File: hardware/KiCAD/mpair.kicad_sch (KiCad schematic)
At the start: 26 parts, among them J3 DX07S016JA1R1500, J4 ARJP11A-MASA-B-A-EMU2, U1 USBLC6-2SC6

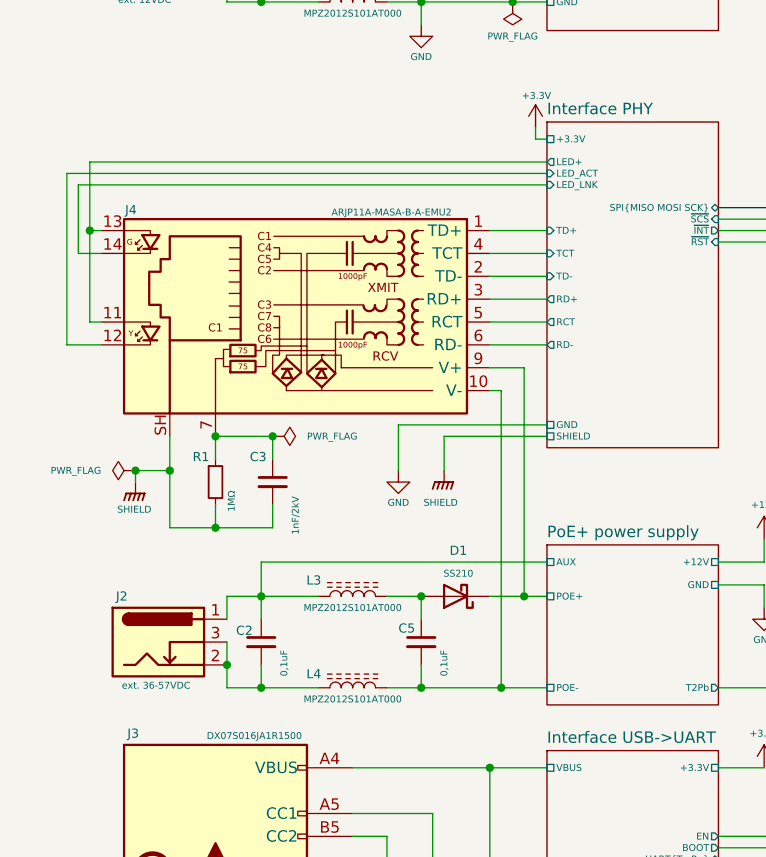
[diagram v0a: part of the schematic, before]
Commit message: update
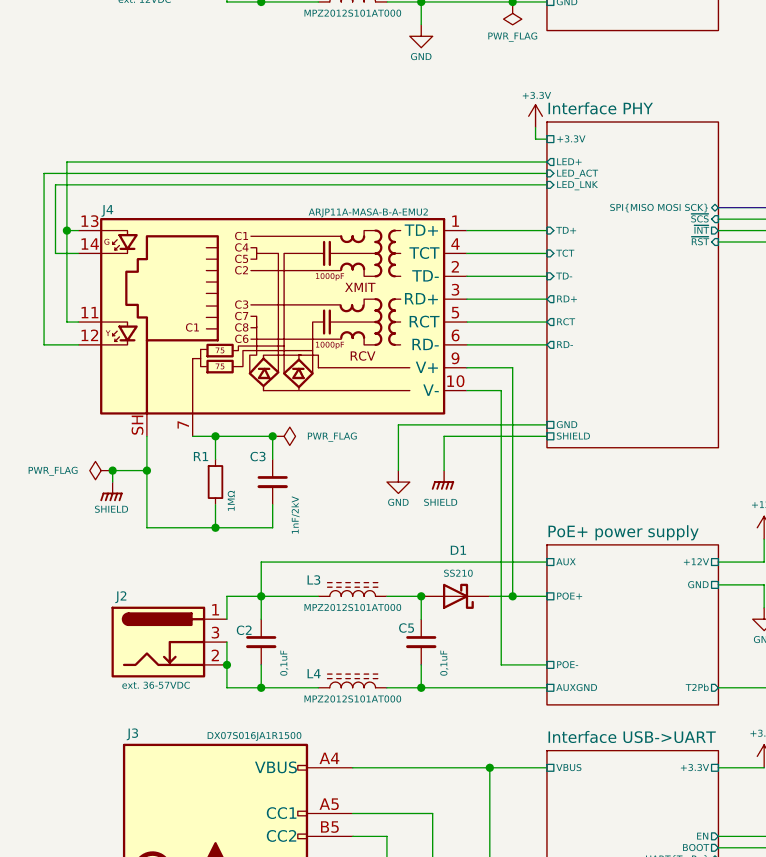
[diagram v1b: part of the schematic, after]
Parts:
- U1: DigiKey_Part_Number (none) -> 5399-USBLC6-2SC6CT-ND; Manufacturer_Name (none) -> USBLC6-2SC6; Manufacturer_Part_Number (none) -> Shenzhen Slkormicro Semicon Co., Ltd.; PACKAGE (none) -> SOT-23-6; Part name USBLC6-2SC6 -> (none)
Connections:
- net PoE+ power supply/POE-: no longer C5.2, L4.2
- new net PoE+ power supply/AUXGND: C5.2, L4.2
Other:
- sheet PoE+ power supply ports: added AUXGND; removed none
- moved on the sheet: J4
